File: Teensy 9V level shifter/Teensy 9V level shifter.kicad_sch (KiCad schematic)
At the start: 47 parts, among them J1 PSU, J10 VGG, J2 TeensyL, J3 CLK, J4 ¬CLK, J5 TeensyR, J6 TeensyL1, J7 TeensyR1, J8 PSU, J9 VCA_CV, SW1 Teensy Vin, U1 4069, U2 4010, U3 LM324, U4 AD5328BRUZ-REEL, U5 TL431DBZ, U6 MCP1826-ADJE/AT

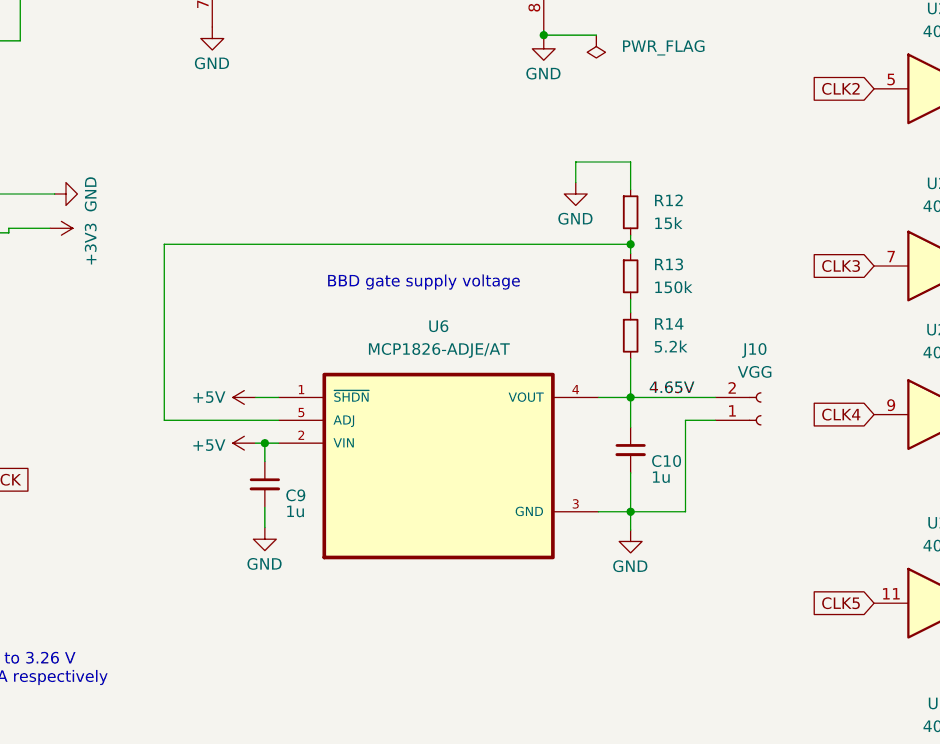
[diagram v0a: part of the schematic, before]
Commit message: Strin Maschine - first revision before review
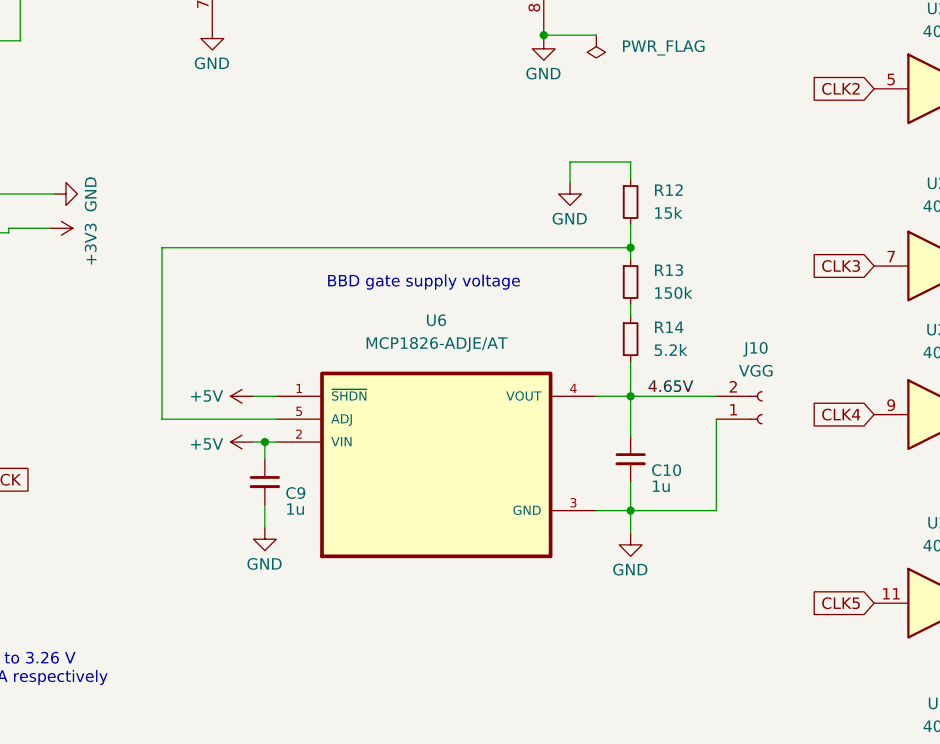
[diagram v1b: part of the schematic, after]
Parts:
- U6: footprint Package_TO_SOT_SMD:SOT-223-6 -> TO170P1066X482X1572-5
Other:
- moved on the sheet: C10, R12, R13
